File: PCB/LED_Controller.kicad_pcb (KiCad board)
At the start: 2 copper layers, 89.5 x 60.5 mm, 97 parts, among them J1 Barrel_Jack, J2 Conn_01x06_Female, J3 74984104400, J4 Screw_Terminal_01x02, J5 Screw_Terminal_01x04, U1 ESP32-PICO-D4, U2 AP62200WU-7, U3 TPS2372, U4 74LVCH2T45DC, U5 LAN8720A, U6 MCP1792x-5002xCB, U7 VCB4805SBO-50WR3, Y1 ECS-250-20-33-CKM-TR

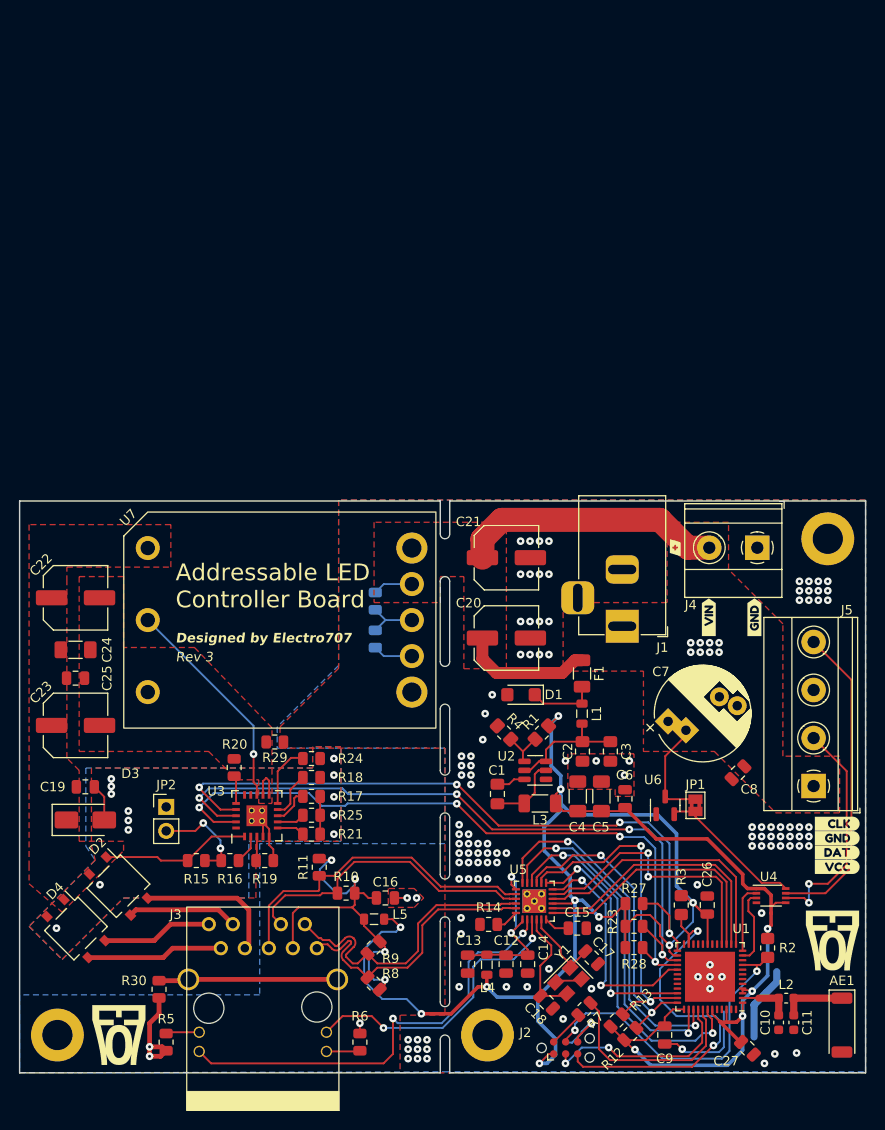
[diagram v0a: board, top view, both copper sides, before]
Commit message: Updated to Rev 4
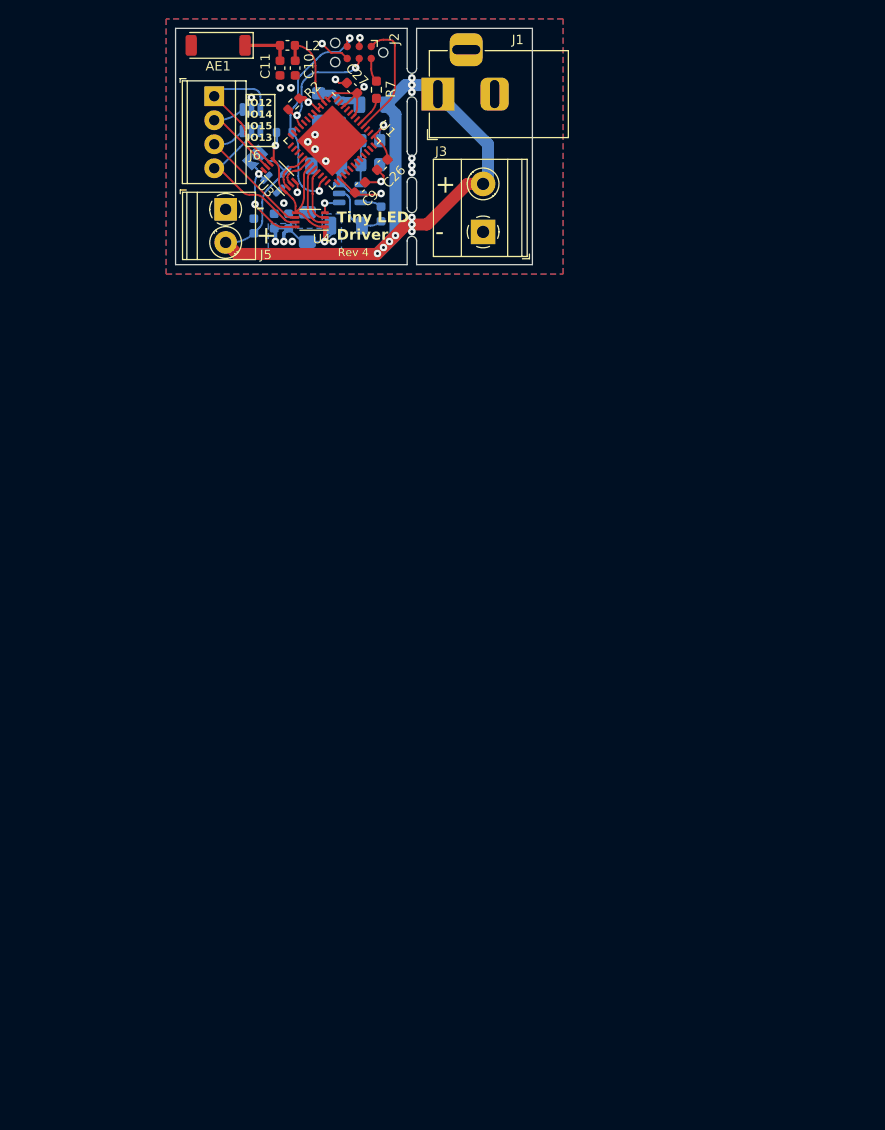
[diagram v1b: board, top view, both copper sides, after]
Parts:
- removed C12, C13, C14, C15, C16: 1uF, Capacitor_SMD:C_0805_2012Metric
- removed C18: C, Capacitor_SMD:C_0805_2012Metric
- removed C19, C25: 0.1u, Capacitor_SMD:C_0805_2012Metric
- removed C20: 330uF, Capacitor_SMD:C_Elec_6.3x5.4
- removed C21: 0.1u, Capacitor_SMD:C_Elec_6.3x5.4
- removed C22: 100uF, Capacitor_SMD:C_Elec_6.3x5.4
- removed C23: 100uF, Capacitor_SMD:C_Elec_6.3x5.8
- removed C24: 1uF, Capacitor_SMD:C_1206_3216Metric_Pad1.33x1.80mm_HandSolder
- removed C4: 10uF, Capacitor_SMD:C_1206_3216Metric_Pad1.33x1.80mm_HandSolder
- removed C7: 1000uF, Capacitor_THT:CP_Radial_D10.0mm_P5.00mm_P7.50mm
- removed D3: SMAJ58A, Diode_SMD:D_SMA
- removed D4: CDBHM220L, Package_TO_SOT_SMD:TO-269AA
- removed G*** (x4): LOGO, LOGO
- removed H1, H2, H3: MountingHole_Pad, MountingHole:MountingHole_3.2mm_M3_DIN965_Pad
- removed J4: Screw_Terminal_01x02, TerminalBlock_Phoenix:TerminalBlock_Phoenix_MKDS-1,5-2-5.08_1x02_P5.08mm_Horizontal
- removed JP2: Jumper_2_Bridged, Connector_PinHeader_2.54mm:PinHeader_1x02_P2.54mm_Vertical
- removed L4, L5: L_Ferrite, Inductor_SMD:L_0805_2012Metric
- removed R10, R11, R8, R9: 49.9, Resistor_SMD:R_0805_2012Metric
- removed R12, R13, R23, R27, R28: 10k, Resistor_SMD:R_0805_2012Metric
- removed R14: 12.1k, Resistor_SMD:R_0805_2012Metric
- removed R15, R16, R17, R18, R19, R21, R22, R24, R25, R26: R, Resistor_SMD:R_0805_2012Metric
- removed R20, R29, R30: 0, Resistor_SMD:R_0805_2012Metric
- removed R5, R6: 1k, Resistor_SMD:R_0805_2012Metric
- removed U6: MCP1792x-5002xCB, Package_TO_SOT_SMD:SOT-23
- removed U7: VCB4805SBO-50WR3, ProjectFootprints:VCB4805SBO-50WR3
- removed Y1: ECS-250-20-33-CKM-TR, Crystal:Crystal_SMD_3225-4Pin_3.2x2.5mm
- removed kibuzzard-64D45D66: G***, kibuzzard-64D45D66
- removed kibuzzard-64D45D6B: G***, kibuzzard-64D45D6B
- removed kibuzzard-64D45DB0: G***, kibuzzard-64D45DB0
- removed kibuzzard-64D45DB7: G***, kibuzzard-64D45DB7
- removed kibuzzard-64D45DBB: G***, kibuzzard-64D45DBB
- removed kibuzzard-64D45DC1: G***, kibuzzard-64D45DC1
- removed kibuzzard-64D45DDA: G***, kibuzzard-64D45DDA
- added J6: Screw_Terminal_01x04, TerminalBlock_TE-Connectivity:TerminalBlock_TE_282834-4_1x04_P2.54mm_Horizontal, F.Cu at (69.1, 75.2)
- C1, C2: footprint Capacitor_SMD:C_0805_2012Metric_Pad1.18x1.45mm_HandSolder -> Capacitor_SMD:C_0603_1608Metric; moved to B.Cu
- C17: value C -> 0.1u; footprint Capacitor_SMD:C_0805_2012Metric -> Capacitor_SMD:C_0603_1608Metric; moved to B.Cu
- C26, C27, C9: footprint Capacitor_SMD:C_0805_2012Metric -> Capacitor_SMD:C_0603_1608Metric
- C3: value 10uF -> 22uF; footprint Capacitor_SMD:C_0805_2012Metric_Pad1.18x1.45mm_HandSolder -> Capacitor_SMD:C_1206_3216Metric_Pad1.33x1.80mm_HandSolder; moved to B.Cu
- C5, D1, F1, L1, L3, R1, R4, U2: moved to B.Cu
- C6, C8: footprint Capacitor_SMD:C_0805_2012Metric -> Capacitor_SMD:C_0603_1608Metric; moved to B.Cu
- D2: value CDBHM220L -> SP0505BAHT; footprint Package_TO_SOT_SMD:TO-269AA -> Package_TO_SOT_SMD:SOT-23-6; moved to B.Cu
- J3: value 74984104400 -> Screw_Terminal_01x02; footprint ProjectFootprints:74984104400 -> TerminalBlock_Phoenix:TerminalBlock_Phoenix_MKDS-1,5-2-5.08_1x02_P5.08mm_Horizontal
- J5: value Screw_Terminal_01x04 -> Screw_Terminal_01x02; footprint TerminalBlock_Phoenix:TerminalBlock_Phoenix_MKDS-1,5-4-5.08_1x04_P5.08mm_Horizontal -> TerminalBlock_Phoenix:TerminalBlock_Phoenix_PT-1,5-2-3.5-H_1x02_P3.50mm_Horizontal
- JP1: footprint Jumper:SolderJumper-2_P1.3mm_Bridged2Bar_Pad1.0x1.5mm -> Jumper:SolderJumper-2_P1.3mm_Open_TrianglePad1.0x1.5mm; moved to B.Cu
- R2: footprint Resistor_SMD:R_0805_2012Metric_Pad1.20x1.40mm_HandSolder -> Resistor_SMD:R_0603_1608Metric
- R3: footprint Resistor_SMD:R_0805_2012Metric_Pad1.20x1.40mm_HandSolder -> Resistor_SMD:R_0603_1608Metric; moved to B.Cu
- R7: footprint Resistor_SMD:R_0805_2012Metric -> Resistor_SMD:R_0603_1608Metric_Pad0.98x0.95mm_HandSolder
- U3: value TPS2372 -> 74LVCH2T45DC; footprint ProjectFootprints:TI_RGW0020B -> Package_SO:VSSOP-8_2.3x2mm_P0.5mm
- U5: value LAN8720A -> MCP1792x-5002xCB; footprint Package_DFN_QFN:VQFN-24-1EP_4x4mm_P0.5mm_EP2.5x2.5mm_ThermalVias -> Package_TO_SOT_SMD:SOT-23; moved to B.Cu
- moved AE1 122.9 mm to (69.5, 69.8), turned to 180 degrees
- moved C11 114.7 mm to (76.0, 72.2)
- moved L2 113.8 mm to (76.8, 69.8), turned to 180 degrees
- moved C10 113.2 mm to (77.7, 72.2)
- moved C27 109.9 mm to (83.7, 74.3), turned to 135 degrees
- moved J2 107.6 mm to (84.4, 70.6), turned to 180 degrees
- moved R2 102.4 mm to (77.5, 76.0), turned to -135 degrees
- moved R7 99.7 mm to (86.2, 74.5), turned to 90 degrees
- moved U1 97.0 mm to (81.6, 79.9), turned to -45 degrees
- moved C9 95.3 mm to (84.5, 84.8), turned to 45 degrees
- moved R3 91.9 mm to (76.5, 79.0), turned to 0 degrees
- moved J5 87.1 mm to (70.3, 87.2), turned to -90 degrees
- moved U4 86.5 mm to (79.2, 88.3), turned to 180 degrees
- moved C26 85.5 mm to (86.9, 82.4), turned to -135 degrees
- moved J3 85.4 mm to (97.5, 89.5), turned to 90 degrees
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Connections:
- C17 pad 1: GND -> +3V3
- C17 pad 2: Net-(U5-XTAL1/CLKIN) -> GND
- D2 pad 1: Net-(D2-+) -> /LED2-CLK_{H}
- D2 pad 2: Net-(D2--) -> GND
- D2 pad 3: /Ethernet and Connector/ETH_V1- -> /LED2-DATA_{H}
- D2 pad 4: /Ethernet and Connector/ETH_V1+ -> unconnected-(D2-K-Pad4)
- J2 pad 1: +3V3 -> /RX
- J2 pad 3: /RX -> +3V3
- J3 pad 1: /Ethernet and Connector/ETH_TX+ -> GND
- J3 pad 2: /Ethernet and Connector/ETH_TX- -> VIN
- J5 pad 1: VIN -> GND
- J5 pad 2: /LED1-DATA_{H} -> VIN
- U1 pad 11: /LED1-DATA_{L} -> unconnected-(U1-IO35-Pad11)
- U1 pad 12: /LED1-CLK_{L} -> unconnected-(U1-IO32-Pad12)
- U1 pad 13: /E_RXER -> unconnected-(U1-IO33-Pad13)
- U1 pad 14: /E_RXD0 -> unconnected-(U1-IO25-Pad14)
- U1 pad 15: /E_RXD1 -> unconnected-(U1-IO26-Pad15)
- U1 pad 16: /E_CRS -> unconnected-(U1-IO27-Pad16)
- U1 pad 17: unconnected-(U1-IO14-Pad17) -> /LED2-CLK_{L}
- U1 pad 18: unconnected-(U1-IO12-Pad18) -> /LED2-DATA_{L}
- U1 pad 20: unconnected-(U1-IO13-Pad20) -> /LED1-CLK_{L}
- U1 pad 21: unconnected-(U1-IO15-Pad21) -> /LED1-DATA_{L}
- U1 pad 25: /POE_TPH -> unconnected-(U1-IO16-Pad25)
- U1 pad 27: /POE_~{BT} -> unconnected-(U1-IO17-Pad27)
- U1 pad 28: /POE_TPL -> unconnected-(U1-SD2/IO9-Pad28)
- U1 pad 29: /E_MDIO -> unconnected-(U1-SD3/IO10-Pad29)
- U1 pad 34: /E_MDC -> unconnected-(U1-IO5-Pad34)
- U1 pad 35: /E_~{INT} -> unconnected-(U1-IO18-Pad35)
- U1 pad 36: /E_~{RST} -> unconnected-(U1-IO23-Pad36)
- U1 pad 38: /E_TXD0 -> unconnected-(U1-IO19-Pad38)
- U1 pad 39: /E_TXD1 -> unconnected-(U1-IO22-Pad39)
- U1 pad 42: /E_TXEN -> unconnected-(U1-IO21-Pad42)
- U3 pad 1: Net-(D2-+) -> +3V3
- U3 pad 2: Net-(U3-DEN) -> /LED2-CLK_{L}
- U3 pad 3: Net-(U3-CLSA) -> /LED2-DATA_{L}
- U3 pad 4: Net-(D2--) -> GND
- U3 pad 5: Net-(D2--) -> +3V3
- U3 pad 6: Net-(U3-CLSB) -> /LED2-DATA_{H}
- U3 pad 7: Net-(U3-REF) -> /LED2-CLK_{H}
- U3 pad 8: Net-(U3-AMPS_CTL) -> +5V
- U5 pad 1: Vdda2 -> GND
- U5 pad 2: /Ethernet and Connector/ETH_LED2 -> +5V
- U5 pad 3: /Ethernet and Connector/ETH_LED1 -> VIN
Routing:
- net +3V3: track 231.2 -> 55.3 mm, vias 14 -> 11
- net /POE_TPH: track 74.7 -> 0.00 mm, vias 4 -> 0
- net /POE_~{BT}: track 74.0 -> 0.00 mm, vias 4 -> 0
- net /POE_TPL: track 72.6 -> 0.00 mm, vias 4 -> 0
- net /Ethernet and Connector/ETH_LED2: track 46.9 -> 0.00 mm, vias 2 -> 0
- net /E_TXEN: track 38.7 -> 0.00 mm, vias 2 -> 0
- net Net-(J3-CD): track 38.2 -> 0.00 mm, vias 4 -> 0
- net /E_TXD1: track 37.8 -> 0.00 mm, vias 2 -> 0
- net /E_TXD0: track 36.7 -> 0.00 mm, vias 2 -> 0
- net /E_~{INT}: track 35.9 -> 0.00 mm, vias 2 -> 0
- net /Ethernet and Connector/ETH_RX-: track 35.3 -> 0.00 mm
- net /E_~{RST}: track 32.7 -> 0.00 mm, vias 2 -> 0
- net /Ethernet and Connector/ETH_TX-: track 32.3 -> 0.00 mm
- net /Ethernet and Connector/ETH_RX+: track 32.3 -> 0.00 mm
- net /Ethernet and Connector/ETH_LED1: track 31.0 -> 0.00 mm, vias 2 -> 0
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- added copper zone on B.Cu, net +3V3
- added copper zone on In2.Cu, net +3V3
- added copper zone on In1.Cu, net GND
- removed copper zone on F.Cu, net Net-(D2-+)
- removed copper zone on B.Cu, net Net-(D2--)
- removed copper zone on F.Cu, net Net-(D2--)
- removed copper zone on F.Cu, net Net-(U7-GND)
- removed copper zone on F.Cu, net VIN
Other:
- board size 89.5 x 60.5 mm -> 37.8 x 25 mm
- copper layers 2 -> 4
- board text added: "+"
- board text added: "-"
- board text added: "IO12"
- board text added: "IO12 IO14 IO15 IO13"
- board text added: "IO13"
- board text added: "IO14"
- board text added: "IO15"
- board text added: "Rev 4"
- board text added: "Tiny LED Driver"
- board text removed: "Addressable LED Controller Board"
- board text removed: "Main Driver Side"
- board text removed: "POE Side"
- board text removed: "Rev 3"
